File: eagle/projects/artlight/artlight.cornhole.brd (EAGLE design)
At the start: 58.4 x 58.4 mm, 28 parts, among them T1 2N2222, T2 2N2222, T3 2N2222, T4 2N2222, T5 2N2222, T6 2N2222, T7 2N2222, T8 2N2222, T9 2N2222

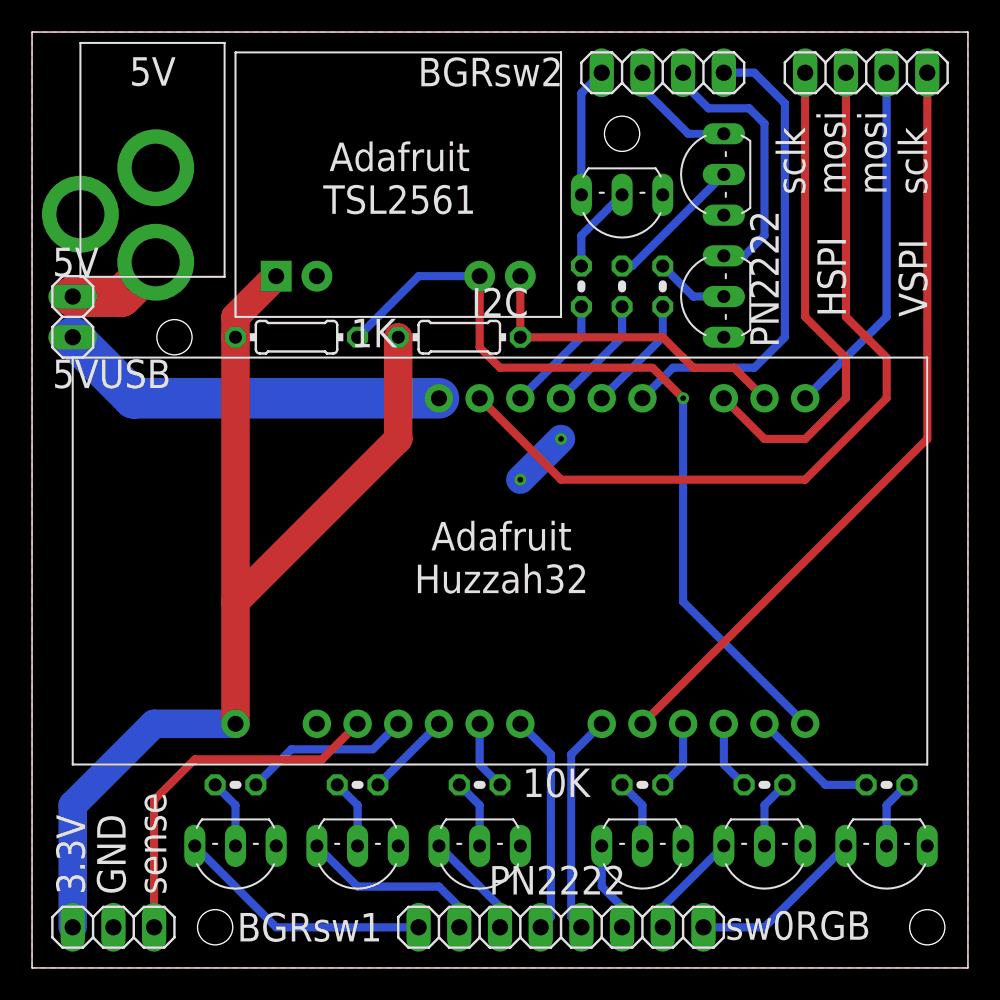
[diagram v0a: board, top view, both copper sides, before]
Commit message: eagle: artlight.cornhole, pins
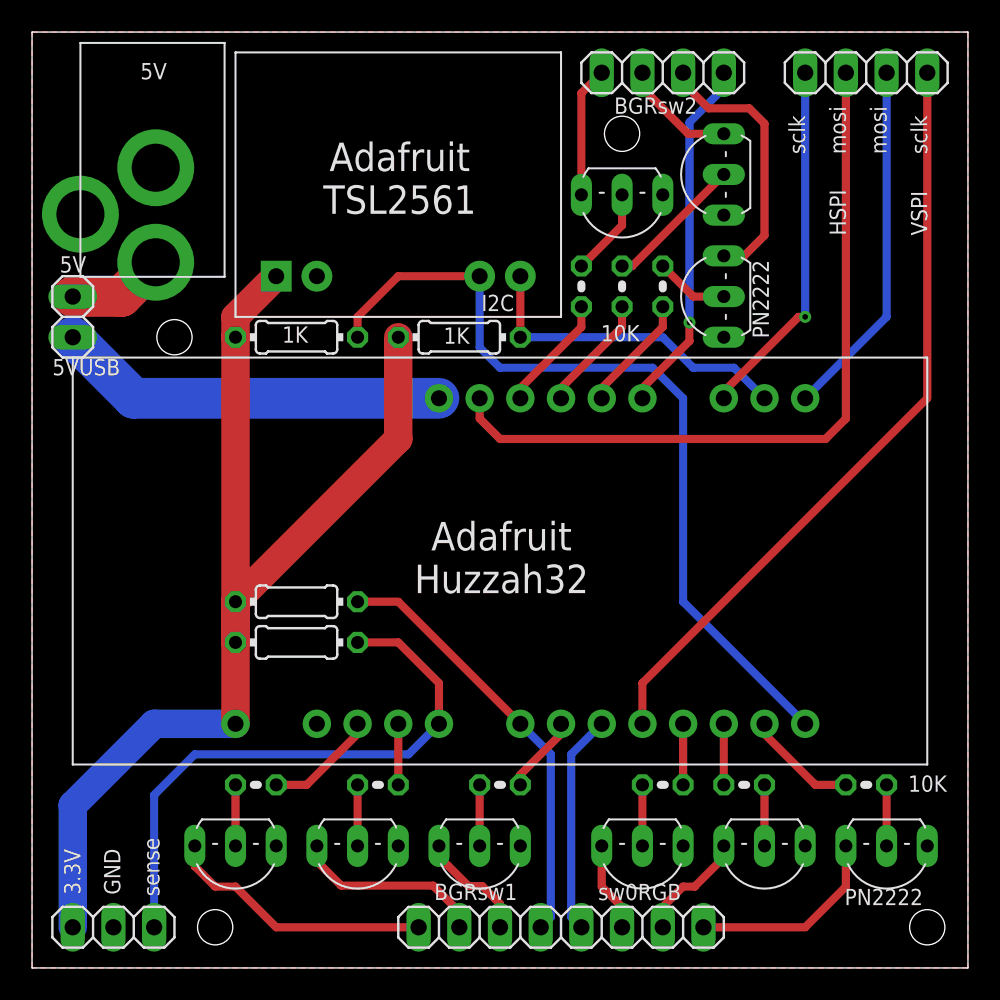
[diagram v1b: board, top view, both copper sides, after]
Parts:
- added R12, R13: 47K, rcl:0204/7
- moved R3 1.27 mm to (52.1, 11.4)
- moved R8 1.27 mm to (14.0, 11.4)
- moved R6 1.27 mm to (29.2, 11.4)
- moved R7 1.27 mm to (21.6, 11.4)
- moved R4 1.27 mm to (44.5, 11.4)
- moved R5 1.27 mm to (39.4, 11.4)
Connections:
- net +3V3: now also R12.2, R13.2
- net SW1: now also R12.1
- net SWBB: now also R13.1
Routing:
- net SWBB: track 22.6 -> 36.5 mm
- net SW1: track 13.8 -> 27.1 mm
- net HSPI-SCLK: track 31.1 -> 22.7 mm, vias 0 -> 1
- net SW2: track 29.7 -> 22.4 mm, vias 0 -> 1
- net HSPI-MOSI: track 51.0 -> 46.8 mm
- net GND: track 3.59 -> 0.00 mm, vias 2 -> 0
- net LED1B: track 10.5 -> 7.03 mm
- net +3V3: track 69.6 -> 72.1 mm
- net LED1G: track 5.39 -> 3.81 mm
- net LED0B-PIN: track 11.0 -> 12.5 mm
- net LED0B: track 7.93 -> 7.03 mm
- net I2C-SDA: track 51.1 -> 51.9 mm, vias 1 -> 0
- net LED1B-PIN: track 16.1 -> 16.8 mm
- net LED0R-BASE: track 4.34 -> 3.81 mm
- net LED0R: track 4.34 -> 3.81 mm
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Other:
- board text added: "LED Switch"
- board text added: "LED Switches"
- board text removed: "(BGRsw2) LED Switches (sw1RGB)"
- board text removed: "LED Switch (sw2RGB)"
